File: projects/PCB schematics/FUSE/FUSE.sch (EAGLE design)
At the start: 26 parts

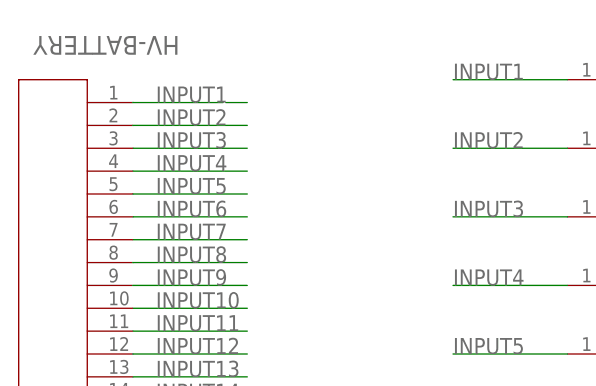
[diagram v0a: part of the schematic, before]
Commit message: PROJ - Gerber files major milestone - 05/05/19.
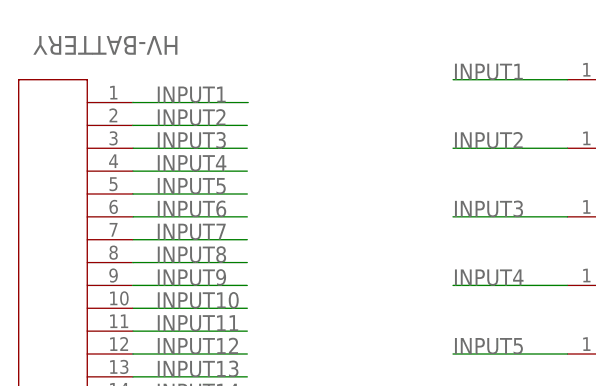
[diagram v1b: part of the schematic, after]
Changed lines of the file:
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@@
 <segment>
 <label x="20.32" y="91.44" size="1.778" layer="95"/>
-<wire x1="27.7876" y1="91.44" x2="17.78" y2="91.44" width="0.1524" layer="91"/>
+<wire x1="30.5816" y1="91.44" x2="17.78" y2="91.44" width="0.1524" layer="91"/>
 <pinref part="HV-BATTERY" gate="A" pin="1"/>
 </segment>
@@
 </segment>
 </net>
-<net name="N$48" class="0">
-<segment>
-<wire x1="30.48" y1="91.44" x2="28.0924" y2="91.44" width="0.1524" layer="91"/>
-</segment>
-</net>
